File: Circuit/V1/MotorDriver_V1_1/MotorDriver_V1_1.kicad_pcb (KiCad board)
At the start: 2 copper layers, 25 x 25 mm, 16 parts, among them J1 Conn_01x04, J2 Conn_01x06_Pin, J3 Conn_01x06_Pin, J4 Conn_01x02, J5 Conn_01x02, J6 Conn_01x02, U1 AM2837, U2 AM2837

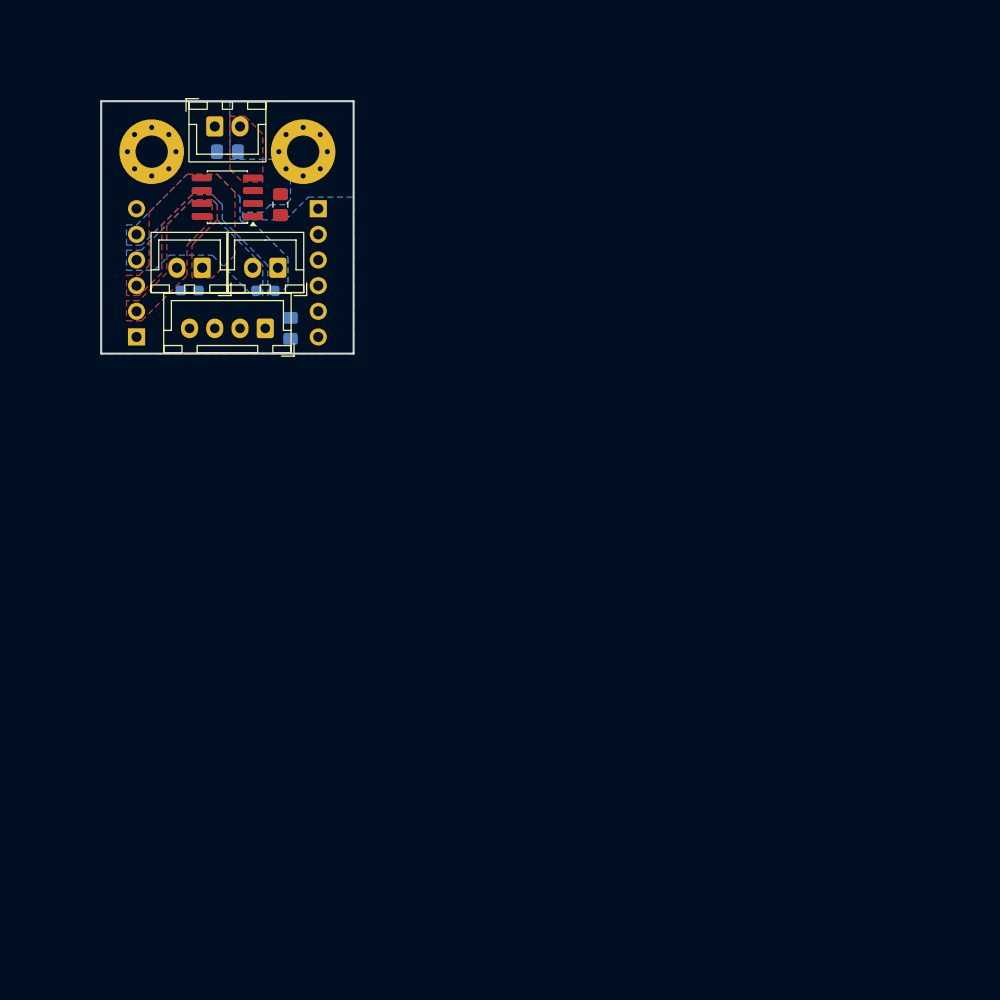
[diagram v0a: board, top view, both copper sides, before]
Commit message: 発注
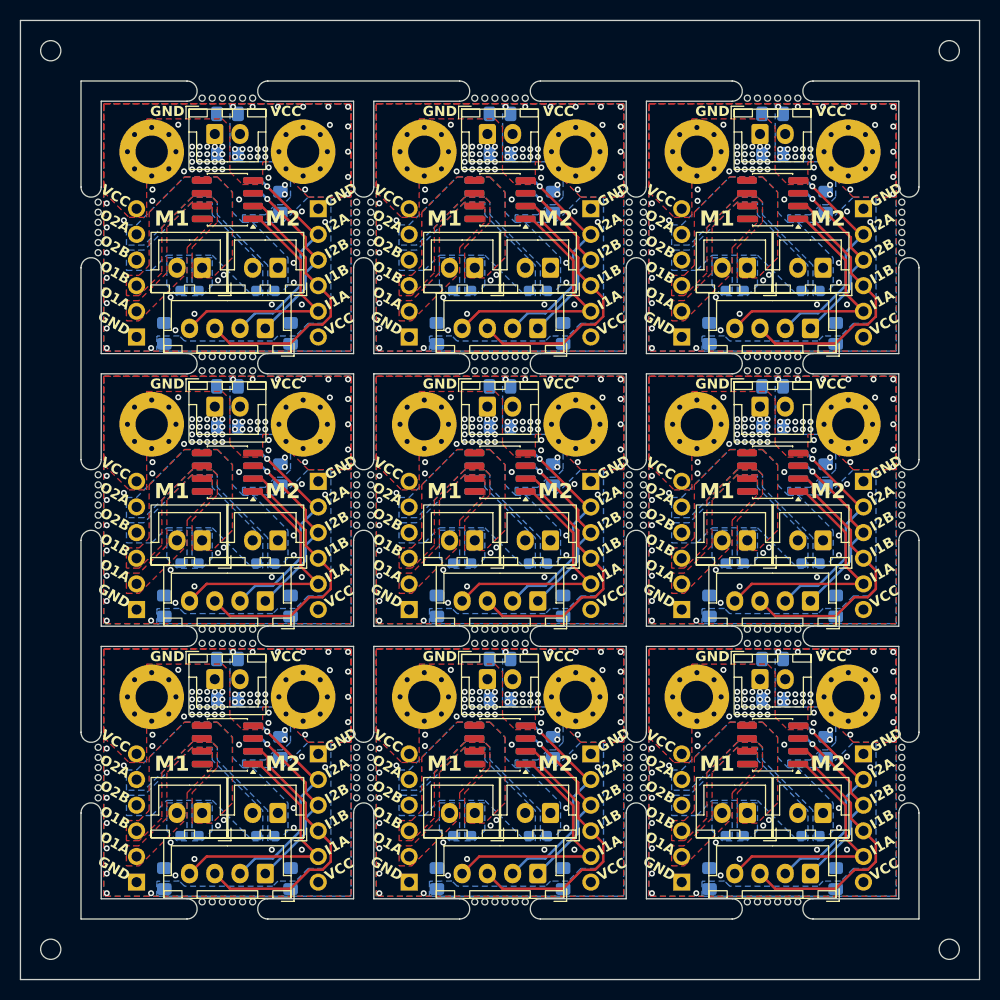
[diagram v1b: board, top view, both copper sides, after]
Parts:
- added C1: 0.1u, Capacitor_SMD:C_0603_1608Metric_Pad1.08x0.95mm_HandSolder, B.Cu at (50.2, 18.8)
- added C1: 0.1u, Capacitor_SMD:C_0603_1608Metric_Pad1.08x0.95mm_HandSolder, B.Cu at (50.3, 45.7)
- added C1: 0.1u, Capacitor_SMD:C_0603_1608Metric_Pad1.08x0.95mm_HandSolder, B.Cu at (50.3, 72.8)
- added C1: 0.1u, Capacitor_SMD:C_0603_1608Metric_Pad1.08x0.95mm_HandSolder, B.Cu at (-3.75, 72.8)
- added C1: 0.1u, Capacitor_SMD:C_0603_1608Metric_Pad1.08x0.95mm_HandSolder, B.Cu at (23.3, 45.7)
- added C1: 0.1u, Capacitor_SMD:C_0603_1608Metric_Pad1.08x0.95mm_HandSolder, B.Cu at (-3.75, 45.7)
- added C1: 0.1u, Capacitor_SMD:C_0603_1608Metric_Pad1.08x0.95mm_HandSolder, B.Cu at (23.3, 72.8)
- added C1: 0.1u, Capacitor_SMD:C_0603_1608Metric_Pad1.08x0.95mm_HandSolder, B.Cu at (23.2, 18.8)
- added C2: 0.1u, Capacitor_SMD:C_0603_1608Metric_Pad1.08x0.95mm_HandSolder, B.Cu at (30.8, 18.8)
- added C2: 0.1u, Capacitor_SMD:C_0603_1608Metric_Pad1.08x0.95mm_HandSolder, B.Cu at (30.8, 45.7)
- added C2: 0.1u, Capacitor_SMD:C_0603_1608Metric_Pad1.08x0.95mm_HandSolder, B.Cu at (3.75, 45.7)
- added C2: 0.1u, Capacitor_SMD:C_0603_1608Metric_Pad1.08x0.95mm_HandSolder, B.Cu at (57.8, 18.8)
- added C2: 0.1u, Capacitor_SMD:C_0603_1608Metric_Pad1.08x0.95mm_HandSolder, B.Cu at (30.8, 72.8)
- added C2: 0.1u, Capacitor_SMD:C_0603_1608Metric_Pad1.08x0.95mm_HandSolder, B.Cu at (3.75, 72.8)
- added C2: 0.1u, Capacitor_SMD:C_0603_1608Metric_Pad1.08x0.95mm_HandSolder, B.Cu at (57.8, 45.7)
- added C2: 0.1u, Capacitor_SMD:C_0603_1608Metric_Pad1.08x0.95mm_HandSolder, B.Cu at (57.8, 72.8)
- added C3: 10u, Capacitor_SMD:C_0805_2012Metric_Pad1.18x1.45mm_HandSolder, B.Cu at (60.3, 50.0)
- added C3: 10u, Capacitor_SMD:C_0805_2012Metric_Pad1.18x1.45mm_HandSolder, B.Cu at (6.25, 77.0)
- added C3: 10u, Capacitor_SMD:C_0805_2012Metric_Pad1.18x1.45mm_HandSolder, B.Cu at (60.2, 23.0)
- added C3: 10u, Capacitor_SMD:C_0805_2012Metric_Pad1.18x1.45mm_HandSolder, B.Cu at (33.3, 50.0)
- added C3: 10u, Capacitor_SMD:C_0805_2012Metric_Pad1.18x1.45mm_HandSolder, B.Cu at (33.3, 77.0)
- added C3: 10u, Capacitor_SMD:C_0805_2012Metric_Pad1.18x1.45mm_HandSolder, B.Cu at (6.25, 50.0)
- added C3: 10u, Capacitor_SMD:C_0805_2012Metric_Pad1.18x1.45mm_HandSolder, B.Cu at (60.3, 77.0)
- added C3: 10u, Capacitor_SMD:C_0805_2012Metric_Pad1.18x1.45mm_HandSolder, B.Cu at (33.2, 23.0)
- added C4: 10u, Capacitor_SMD:C_0805_2012Metric_Pad1.18x1.45mm_HandSolder, B.Cu at (27.0, 5.25)
- added C4: 10u, Capacitor_SMD:C_0805_2012Metric_Pad1.18x1.45mm_HandSolder, B.Cu at (0.00, 32.2)
- added C4: 10u, Capacitor_SMD:C_0805_2012Metric_Pad1.18x1.45mm_HandSolder, B.Cu at (27.0, 59.3)
- added C4: 10u, Capacitor_SMD:C_0805_2012Metric_Pad1.18x1.45mm_HandSolder, B.Cu at (54.0, 32.2)
- added C4: 10u, Capacitor_SMD:C_0805_2012Metric_Pad1.18x1.45mm_HandSolder, B.Cu at (0.00, 59.3)
- added C4: 10u, Capacitor_SMD:C_0805_2012Metric_Pad1.18x1.45mm_HandSolder, B.Cu at (54.0, 59.3)
- added C4: 10u, Capacitor_SMD:C_0805_2012Metric_Pad1.18x1.45mm_HandSolder, B.Cu at (54.0, 5.25)
- added C4: 10u, Capacitor_SMD:C_0805_2012Metric_Pad1.18x1.45mm_HandSolder, B.Cu at (27.0, 32.2)
- added C5: 10u, Capacitor_SMD:C_0805_2012Metric_Pad1.18x1.45mm_HandSolder, B.Cu at (54.0, 28.2)
- added C5: 10u, Capacitor_SMD:C_0805_2012Metric_Pad1.18x1.45mm_HandSolder, B.Cu at (54.0, 1.25)
- added C5: 10u, Capacitor_SMD:C_0805_2012Metric_Pad1.18x1.45mm_HandSolder, B.Cu at (54.0, 55.3)
- added C5: 10u, Capacitor_SMD:C_0805_2012Metric_Pad1.18x1.45mm_HandSolder, B.Cu at (0.00, 28.2)
- added C5: 10u, Capacitor_SMD:C_0805_2012Metric_Pad1.18x1.45mm_HandSolder, B.Cu at (0.00, 55.3)
- added C5: 10u, Capacitor_SMD:C_0805_2012Metric_Pad1.18x1.45mm_HandSolder, B.Cu at (27.0, 1.25)
- added C5: 10u, Capacitor_SMD:C_0805_2012Metric_Pad1.18x1.45mm_HandSolder, B.Cu at (27.0, 28.2)
- added C5: 10u, Capacitor_SMD:C_0805_2012Metric_Pad1.18x1.45mm_HandSolder, B.Cu at (27.0, 55.3)
- added C6: 10u, Capacitor_SMD:C_0805_2012Metric_Pad1.18x1.45mm_HandSolder, B.Cu at (5.25, 64.0)
- added C6: 10u, Capacitor_SMD:C_0805_2012Metric_Pad1.18x1.45mm_HandSolder, B.Cu at (32.3, 37.0)
- added C6: 10u, Capacitor_SMD:C_0805_2012Metric_Pad1.18x1.45mm_HandSolder, B.Cu at (59.3, 64.0)
- added C6: 10u, Capacitor_SMD:C_0805_2012Metric_Pad1.18x1.45mm_HandSolder, B.Cu at (59.3, 37.0)
- added C6: 10u, Capacitor_SMD:C_0805_2012Metric_Pad1.18x1.45mm_HandSolder, B.Cu at (32.2, 10.0)
- added C6: 10u, Capacitor_SMD:C_0805_2012Metric_Pad1.18x1.45mm_HandSolder, B.Cu at (32.3, 64.0)
- added C6: 10u, Capacitor_SMD:C_0805_2012Metric_Pad1.18x1.45mm_HandSolder, B.Cu at (59.2, 10.0)
- added C6: 10u, Capacitor_SMD:C_0805_2012Metric_Pad1.18x1.45mm_HandSolder, B.Cu at (5.25, 37.0)
- added C7: 10u, Capacitor_SMD:C_0805_2012Metric_Pad1.18x1.45mm_HandSolder, B.Cu at (-6.25, 23.0)
- added C7: 10u, Capacitor_SMD:C_0805_2012Metric_Pad1.18x1.45mm_HandSolder, B.Cu at (47.8, 23.0)
- added C7: 10u, Capacitor_SMD:C_0805_2012Metric_Pad1.18x1.45mm_HandSolder, B.Cu at (20.8, 50.0)
- added C7: 10u, Capacitor_SMD:C_0805_2012Metric_Pad1.18x1.45mm_HandSolder, B.Cu at (20.8, 77.0)
- added C7: 10u, Capacitor_SMD:C_0805_2012Metric_Pad1.18x1.45mm_HandSolder, B.Cu at (47.8, 50.0)
- added C7: 10u, Capacitor_SMD:C_0805_2012Metric_Pad1.18x1.45mm_HandSolder, B.Cu at (-6.25, 50.0)
- added C7: 10u, Capacitor_SMD:C_0805_2012Metric_Pad1.18x1.45mm_HandSolder, B.Cu at (-6.25, 77.0)
- added C7: 10u, Capacitor_SMD:C_0805_2012Metric_Pad1.18x1.45mm_HandSolder, B.Cu at (47.8, 77.0)
- added C7: 10u, Capacitor_SMD:C_0805_2012Metric_Pad1.18x1.45mm_HandSolder, B.Cu at (20.8, 23.0)
- added H1: MountingHole, MountingHole:MountingHole_3.2mm_M3_Pad_Via, F.Cu at (19.5, 32.0)
- added H1: MountingHole, MountingHole:MountingHole_3.2mm_M3_Pad_Via, F.Cu at (-7.50, 32.0)
- added H1: MountingHole, MountingHole:MountingHole_3.2mm_M3_Pad_Via, F.Cu at (19.5, 59.0)
- added H1: MountingHole, MountingHole:MountingHole_3.2mm_M3_Pad_Via, F.Cu at (46.5, 32.0)
- added H1: MountingHole, MountingHole:MountingHole_3.2mm_M3_Pad_Via, F.Cu at (-7.50, 59.0)
- added H1: MountingHole, MountingHole:MountingHole_3.2mm_M3_Pad_Via, F.Cu at (46.5, 59.0)
- added H1: MountingHole, MountingHole:MountingHole_3.2mm_M3_Pad_Via, F.Cu at (19.5, 5.00)
- added H1: MountingHole, MountingHole:MountingHole_3.2mm_M3_Pad_Via, F.Cu at (46.5, 5.00)
- added H2: MountingHole, MountingHole:MountingHole_3.2mm_M3_Pad_Via, F.Cu at (34.5, 59.0)
- added H2: MountingHole, MountingHole:MountingHole_3.2mm_M3_Pad_Via, F.Cu at (7.50, 32.0)
- added H2: MountingHole, MountingHole:MountingHole_3.2mm_M3_Pad_Via, F.Cu at (61.5, 32.0)
- added H2: MountingHole, MountingHole:MountingHole_3.2mm_M3_Pad_Via, F.Cu at (61.5, 59.0)
- added H2: MountingHole, MountingHole:MountingHole_3.2mm_M3_Pad_Via, F.Cu at (34.5, 5.00)
- added H2: MountingHole, MountingHole:MountingHole_3.2mm_M3_Pad_Via, F.Cu at (7.50, 59.0)
- added H2: MountingHole, MountingHole:MountingHole_3.2mm_M3_Pad_Via, F.Cu at (34.5, 32.0)
- added H2: MountingHole, MountingHole:MountingHole_3.2mm_M3_Pad_Via, F.Cu at (61.5, 5.00)
- added J1: Conn_01x04, Connector_JST:JST_XH_B4B-XH-A_1x04_P2.50mm_Vertical, F.Cu at (57.8, 76.5)
- added J1: Conn_01x04, Connector_JST:JST_XH_B4B-XH-A_1x04_P2.50mm_Vertical, F.Cu at (3.75, 76.5)
- added J1: Conn_01x04, Connector_JST:JST_XH_B4B-XH-A_1x04_P2.50mm_Vertical, F.Cu at (57.8, 22.5)
- added J1: Conn_01x04, Connector_JST:JST_XH_B4B-XH-A_1x04_P2.50mm_Vertical, F.Cu at (30.8, 22.5)
- added J1: Conn_01x04, Connector_JST:JST_XH_B4B-XH-A_1x04_P2.50mm_Vertical, F.Cu at (3.75, 49.5)
- added J1: Conn_01x04, Connector_JST:JST_XH_B4B-XH-A_1x04_P2.50mm_Vertical, F.Cu at (57.8, 49.5)
- added J1: Conn_01x04, Connector_JST:JST_XH_B4B-XH-A_1x04_P2.50mm_Vertical, F.Cu at (30.8, 49.5)
- added J1: Conn_01x04, Connector_JST:JST_XH_B4B-XH-A_1x04_P2.50mm_Vertical, F.Cu at (30.8, 76.5)
- added J2: Conn_01x06_Pin, Connector_PinHeader_2.54mm:PinHeader_1x06_P2.54mm_Vertical, B.Cu at (36.0, 10.7)
- added J2: Conn_01x06_Pin, Connector_PinHeader_2.54mm:PinHeader_1x06_P2.54mm_Vertical, B.Cu at (63.0, 10.7)
- added J2: Conn_01x06_Pin, Connector_PinHeader_2.54mm:PinHeader_1x06_P2.54mm_Vertical, B.Cu at (9.00, 64.7)
- added J2: Conn_01x06_Pin, Connector_PinHeader_2.54mm:PinHeader_1x06_P2.54mm_Vertical, B.Cu at (36.0, 37.6)
- added J2: Conn_01x06_Pin, Connector_PinHeader_2.54mm:PinHeader_1x06_P2.54mm_Vertical, B.Cu at (36.0, 64.7)
- added J2: Conn_01x06_Pin, Connector_PinHeader_2.54mm:PinHeader_1x06_P2.54mm_Vertical, B.Cu at (63.0, 37.6)
- added J2: Conn_01x06_Pin, Connector_PinHeader_2.54mm:PinHeader_1x06_P2.54mm_Vertical, B.Cu at (63.0, 64.7)
- added J2: Conn_01x06_Pin, Connector_PinHeader_2.54mm:PinHeader_1x06_P2.54mm_Vertical, B.Cu at (9.00, 37.6)
- added J3: Conn_01x06_Pin, Connector_PinHeader_2.54mm:PinHeader_1x06_P2.54mm_Vertical, B.Cu at (18.0, 23.4)
- added J3: Conn_01x06_Pin, Connector_PinHeader_2.54mm:PinHeader_1x06_P2.54mm_Vertical, B.Cu at (45.0, 50.3)
- added J3: Conn_01x06_Pin, Connector_PinHeader_2.54mm:PinHeader_1x06_P2.54mm_Vertical, B.Cu at (-9.00, 50.3)
- added J3: Conn_01x06_Pin, Connector_PinHeader_2.54mm:PinHeader_1x06_P2.54mm_Vertical, B.Cu at (18.0, 50.3)
- added J3: Conn_01x06_Pin, Connector_PinHeader_2.54mm:PinHeader_1x06_P2.54mm_Vertical, B.Cu at (-9.00, 77.4)
- added J3: Conn_01x06_Pin, Connector_PinHeader_2.54mm:PinHeader_1x06_P2.54mm_Vertical, B.Cu at (45.0, 23.4)
- added J3: Conn_01x06_Pin, Connector_PinHeader_2.54mm:PinHeader_1x06_P2.54mm_Vertical, B.Cu at (45.0, 77.4)
- added J3: Conn_01x06_Pin, Connector_PinHeader_2.54mm:PinHeader_1x06_P2.54mm_Vertical, B.Cu at (18.0, 77.4)
- added J4: Conn_01x02, Connector_JST:JST_XH_B2B-XH-A_1x02_P2.50mm_Vertical, F.Cu at (24.5, 43.5)
- added J4: Conn_01x02, Connector_JST:JST_XH_B2B-XH-A_1x02_P2.50mm_Vertical, F.Cu at (-2.50, 43.5)
- added J4: Conn_01x02, Connector_JST:JST_XH_B2B-XH-A_1x02_P2.50mm_Vertical, F.Cu at (-2.50, 70.5)
- added J4: Conn_01x02, Connector_JST:JST_XH_B2B-XH-A_1x02_P2.50mm_Vertical, F.Cu at (24.5, 70.5)
- added J4: Conn_01x02, Connector_JST:JST_XH_B2B-XH-A_1x02_P2.50mm_Vertical, F.Cu at (51.5, 43.5)
- added J4: Conn_01x02, Connector_JST:JST_XH_B2B-XH-A_1x02_P2.50mm_Vertical, F.Cu at (24.5, 16.5)
- added J4: Conn_01x02, Connector_JST:JST_XH_B2B-XH-A_1x02_P2.50mm_Vertical, F.Cu at (51.5, 16.5)
- added J4: Conn_01x02, Connector_JST:JST_XH_B2B-XH-A_1x02_P2.50mm_Vertical, F.Cu at (51.5, 70.5)
- added J5: Conn_01x02, Connector_JST:JST_XH_B2B-XH-A_1x02_P2.50mm_Vertical, F.Cu at (25.8, 30.2)
- added J5: Conn_01x02, Connector_JST:JST_XH_B2B-XH-A_1x02_P2.50mm_Vertical, F.Cu at (25.8, 57.3)
- added J5: Conn_01x02, Connector_JST:JST_XH_B2B-XH-A_1x02_P2.50mm_Vertical, F.Cu at (-1.25, 57.3)
- added J5: Conn_01x02, Connector_JST:JST_XH_B2B-XH-A_1x02_P2.50mm_Vertical, F.Cu at (52.8, 30.2)
- added J5: Conn_01x02, Connector_JST:JST_XH_B2B-XH-A_1x02_P2.50mm_Vertical, F.Cu at (-1.25, 30.2)
- added J5: Conn_01x02, Connector_JST:JST_XH_B2B-XH-A_1x02_P2.50mm_Vertical, F.Cu at (25.8, 3.25)
- added J5: Conn_01x02, Connector_JST:JST_XH_B2B-XH-A_1x02_P2.50mm_Vertical, F.Cu at (52.8, 57.3)
- added J5: Conn_01x02, Connector_JST:JST_XH_B2B-XH-A_1x02_P2.50mm_Vertical, F.Cu at (52.8, 3.25)
- added J6: Conn_01x02, Connector_JST:JST_XH_B2B-XH-A_1x02_P2.50mm_Vertical, F.Cu at (32.0, 43.5)
- added J6: Conn_01x02, Connector_JST:JST_XH_B2B-XH-A_1x02_P2.50mm_Vertical, F.Cu at (59.0, 16.5)
- added J6: Conn_01x02, Connector_JST:JST_XH_B2B-XH-A_1x02_P2.50mm_Vertical, F.Cu at (32.0, 16.5)
- added J6: Conn_01x02, Connector_JST:JST_XH_B2B-XH-A_1x02_P2.50mm_Vertical, F.Cu at (59.0, 70.5)
- added J6: Conn_01x02, Connector_JST:JST_XH_B2B-XH-A_1x02_P2.50mm_Vertical, F.Cu at (5.00, 43.5)
- added J6: Conn_01x02, Connector_JST:JST_XH_B2B-XH-A_1x02_P2.50mm_Vertical, F.Cu at (5.00, 70.5)
- added J6: Conn_01x02, Connector_JST:JST_XH_B2B-XH-A_1x02_P2.50mm_Vertical, F.Cu at (32.0, 70.5)
- added J6: Conn_01x02, Connector_JST:JST_XH_B2B-XH-A_1x02_P2.50mm_Vertical, F.Cu at (59.0, 43.5)
- added REF**: Mouse_bites, 0-Library:Mouse_bites, F.Cu at (54.0, 53.0)
- added REF**: Mouse_bites_one_side, 0-Library:Mouse_bites_one_side, F.Cu at (67.5, 66.5)
- added REF**: Mouse_bites, 0-Library:Mouse_bites, F.Cu at (13.5, 12.5)
- added REF**: Mouse_bites_one_side, 0-Library:Mouse_bites_one_side, F.Cu at (67.5, 12.5)
- added REF**: Mouse_bites_one_side, 0-Library:Mouse_bites_one_side, F.Cu at (-13.5, 12.5)
- added REF**: Mouse_bites_one_side, 0-Library:Mouse_bites_one_side, F.Cu at (54.0, 80.0)
- added REF**: Mouse_bites_one_side, 0-Library:Mouse_bites_one_side, F.Cu at (54.0, -1.00)
- added REF**: Mouse_bites_one_side, 0-Library:Mouse_bites_one_side, F.Cu at (-13.5, 66.5)
- added REF**: Mouse_bites, 0-Library:Mouse_bites, F.Cu at (40.5, 66.5)
- added REF**: Mouse_bites_one_side, 0-Library:Mouse_bites_one_side, F.Cu at (0.00, -1.00)
- added REF**: Mouse_bites, 0-Library:Mouse_bites, F.Cu at (54.0, 26.0)
- added REF**: Mouse_bites, 0-Library:Mouse_bites, F.Cu at (40.5, 39.5)
- added REF**: Mouse_bites_one_side, 0-Library:Mouse_bites_one_side, F.Cu at (-13.5, 39.5)
- added REF**: Mouse_bites, 0-Library:Mouse_bites, F.Cu at (0.00, 53.0)
- added REF**: Mouse_bites, 0-Library:Mouse_bites, F.Cu at (40.5, 12.5)
- added REF**: Mouse_bites, 0-Library:Mouse_bites, F.Cu at (13.5, 66.5)
- added REF**: Mouse_bites_one_side, 0-Library:Mouse_bites_one_side, F.Cu at (27.0, 80.0)
- added REF**: Mouse_bites, 0-Library:Mouse_bites, F.Cu at (0.00, 26.0)
- added REF**: Mouse_bites_one_side, 0-Library:Mouse_bites_one_side, F.Cu at (67.5, 39.5)
- added REF**: Mouse_bites, 0-Library:Mouse_bites, F.Cu at (13.5, 39.5)
- added REF**: Mouse_bites, 0-Library:Mouse_bites, F.Cu at (27.0, 26.0)
- added REF**: Mouse_bites_one_side, 0-Library:Mouse_bites_one_side, F.Cu at (0.00, 80.0)
- added REF**: Mouse_bites, 0-Library:Mouse_bites, F.Cu at (27.0, 53.0)
- added REF**: Mouse_bites_one_side, 0-Library:Mouse_bites_one_side, F.Cu at (27.0, -1.00)
- added U1: AM2837, Package_SO:SOP-8_3.76x4.96mm_P1.27mm, F.Cu at (54.0, 63.8)
- added U1: AM2837, Package_SO:SOP-8_3.76x4.96mm_P1.27mm, F.Cu at (27.0, 9.75)
- added U1: AM2837, Package_SO:SOP-8_3.76x4.96mm_P1.27mm, F.Cu at (54.0, 9.75)
- added U1: AM2837, Package_SO:SOP-8_3.76x4.96mm_P1.27mm, F.Cu at (0.00, 63.8)
- added U1: AM2837, Package_SO:SOP-8_3.76x4.96mm_P1.27mm, F.Cu at (0.00, 36.7)
- added U1: AM2837, Package_SO:SOP-8_3.76x4.96mm_P1.27mm, F.Cu at (27.0, 36.7)
- added U1: AM2837, Package_SO:SOP-8_3.76x4.96mm_P1.27mm, F.Cu at (27.0, 63.8)
- added U1: AM2837, Package_SO:SOP-8_3.76x4.96mm_P1.27mm, F.Cu at (54.0, 36.7)
- added U2: AM2837, Package_SO:SOP-8_3.76x4.96mm_P1.27mm, B.Cu at (0.00, 63.8)
- added U2: AM2837, Package_SO:SOP-8_3.76x4.96mm_P1.27mm, B.Cu at (54.0, 36.7)
- added U2: AM2837, Package_SO:SOP-8_3.76x4.96mm_P1.27mm, B.Cu at (27.0, 9.75)
- added U2: AM2837, Package_SO:SOP-8_3.76x4.96mm_P1.27mm, B.Cu at (54.0, 9.75)
- added U2: AM2837, Package_SO:SOP-8_3.76x4.96mm_P1.27mm, B.Cu at (27.0, 63.8)
- added U2: AM2837, Package_SO:SOP-8_3.76x4.96mm_P1.27mm, B.Cu at (27.0, 36.7)
- added U2: AM2837, Package_SO:SOP-8_3.76x4.96mm_P1.27mm, B.Cu at (0.00, 36.7)
- added U2: AM2837, Package_SO:SOP-8_3.76x4.96mm_P1.27mm, B.Cu at (54.0, 63.8)
- C6: moved to B.Cu
- moved C5 10.4 mm to (0.00, 1.25), turned to 0 degrees
- moved J5 0.75 mm to (-1.25, 3.25)
- moved C3 0.50 mm to (6.25, 23.0)
- moved C4 0.25 mm to (0.00, 5.25)
- moved C6 0.25 mm to (5.25, 10.0), turned to -90 degrees
- moved U1 0.25 mm to (0.00, 9.75)
- moved U2 0.25 mm to (0.00, 9.75)
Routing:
- net IN1B: track 0.00 -> 250.4 mm
- net IN1A: track 0.00 -> 230.8 mm
- net IN2A: track 0.00 -> 200.0 mm, vias 0 -> 9
- net IN2B: track 0.00 -> 168.6 mm, vias 0 -> 9
- net VCC: vias 0 -> 198
- net GND: vias 0 -> 441
- added copper zone on B.Cu, net OUT1A
- added copper zone on B.Cu, net OUT1B
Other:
- board size 25 x 25 mm -> 95 x 95 mm
- board text added: "AM2837"
- board text added: "GND"
- board text added: "I1A"
- board text added: "I1B"
- board text added: "I2A"
- board text added: "I2B"
- board text added: "Input 13.5v max"
- board text added: "M1"
- board text added: "M2"
- board text added: "MotorDriver V1.1"
- board text added: "O1A"
- board text added: "O1B"
- board text added: "O2A"
- board text added: "O2B"
- board text added: "VCC"
